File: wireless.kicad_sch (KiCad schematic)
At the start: 36 parts, among them J301 J_TC2030-IDC, Q301 Q_SOT23_NPN, Q302 Q_SOT23_NPN, U301 U_ATGM336H-5N31, U302 U_ESP32-C3-MINI-1U-N4, U303 U_AT2659, U304 U_RA-01S

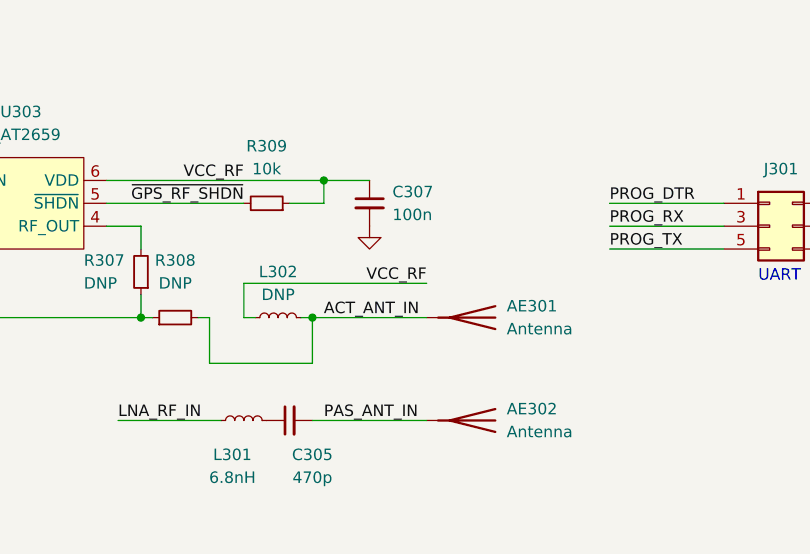
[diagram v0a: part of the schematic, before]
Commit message: production: prepare for fab
Signed-off-by: Connor Rigby <connorr@hey.com>
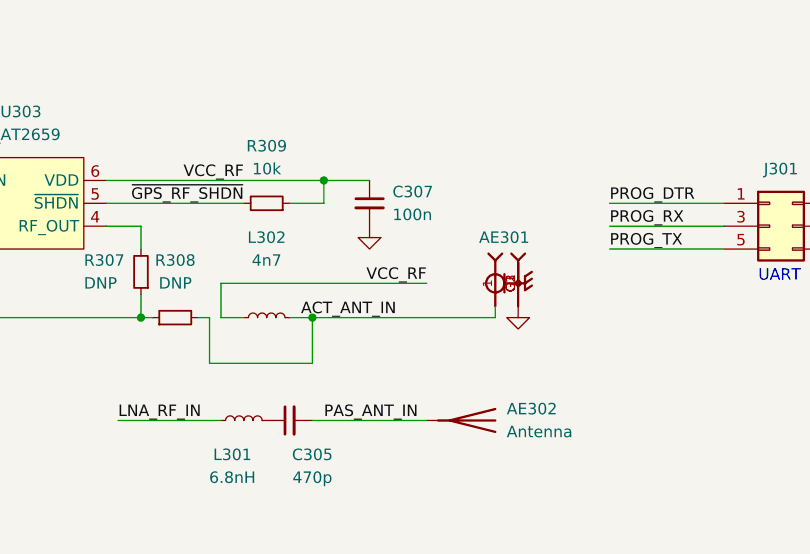
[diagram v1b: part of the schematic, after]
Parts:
- AE301: value Antenna -> 20579-001E; footprint (none) -> BOM:IPEX_20579-001E; symbol Device:Antenna -> BOM:20579-001E; LCSC (none) -> C2987683; MANUFACTURER (none) -> I-PEX; MPN (none) -> IPEX-4
- AE302, C305, C307, L301, R307, R309, U303: now left out of the parts list
- L302: value L_0402_DNP -> L_4n7; symbol BOM:L_0402_DNP -> BOM:L_4n7; Inductance DNP -> 4n7; LCSC (none) -> C13595; MPN (none) -> SDCL1005C4N7STDF
- U302: LCSC C2911374 -> C3013922; MPN ESP32-C3-MINI-1U-N4 -> ESP32-C3-MINI-1U-H4
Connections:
- net GND: now also AE301.G1, AE301.G2, AE301.G3
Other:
- moved on the sheet: L302
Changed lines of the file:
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@@
     (stroke (width 0) (type default) (color 0 0 0 0))
   )
-  (wire (pts (xy 137.16 144.78) (xy 135.89 144.78))
+  (wire (pts (xy 135.89 144.78) (xy 133.35 144.78))
     (stroke (width 0) (type default) (color 0 0 0 0))
   )
@@
     (stroke (width 0) (type default) (color 0 0 0 0))
   )
+  (wire (pts (xy 163.83 143.51) (xy 163.83 144.78))
+    (stroke (width 0) (type default) (color 0 0 0 0))
+  )
   (wire (pts (xy 243.84 67.31) (xy 260.35 67.31))
     (stroke (width 0) (type default) (color 0 0 0 0))
@@
     (stroke (width 0) (type default) (color 0 0 0 0))
   )
-  (wire (pts (xy 142.24 144.78) (xy 143.51 144.78))
+  (wire (pts (xy 140.97 144.78) (xy 143.51 144.78))
     (stroke (width 0) (type default) (color 0 0 0 0))
   )
@@
     (stroke (width 0) (type default) (color 0 0 0 0))
   )
-  (wire (pts (xy 156.21 144.78) (xy 143.51 144.78))
-    (stroke (width 0) (type default) (color 0 0 0 0))
-  )
-  (wire (pts (xy 156.21 140.97) (xy 135.89 140.97))
+  (wire (pts (xy 143.51 144.78) (xy 163.83 144.78))
+    (stroke (width 0) (type default) (color 0 0 0 0))
+  )
+  (wire (pts (xy 156.21 140.97) (xy 133.35 140.97))
     (stroke (width 0) (type default) (color 0 0 0 0))
   )
@@
     (stroke (width 0) (type default) (color 0 0 0 0))
   )
-  (wire (pts (xy 135.89 140.97) (xy 135.89 144.78))
+  (wire (pts (xy 133.35 140.97) (xy 133.35 144.78))
     (stroke (width 0) (type default) (color 0 0 0 0))
   )
@@
     (effects (font (size 1.27 1.27)) (justify left bottom))
   )
-  (label "ACT_ANT_IN" (at 144.78 144.78 0)
+  (label "ACT_ANT_IN" (at 142.24 144.78 0)
     (effects (font (size 1.27 1.27)) (justify left bottom))
   )
@@
   )
   (symbol (lib_id "BOM:R_0402_DNP") (at 124.46 139.7 180) (unit 1)
-    (in_bom yes) (on_board yes)
+    (in_bom no) (on_board no)
     (property "Reference" "R307" (id 0) (at 118.11 138.4299 0)
       (effects (font (size 1.27 1.27)) (justify right))
@@
   )
   (symbol (lib_id "Device:Antenna") (at 161.29 156.21 270) (unit 1)
-    (in_bom yes) (on_board yes) (fields_autoplaced)
+    (in_bom no) (on_board no) (fields_autoplaced)
     (property "Reference" "AE302" (id 0) (at 165.1 154.9399 90)
       (effects (font (size 1.27 1.27)) (justify left))
@@
     )
     (property "Datasheet" "" (id 3) (at 57.15 162.56 0)
+      (effects (font (size 1.27 1.27)) hide)
+    )
+    (pin "1")
+  )
+  (symbol (lib_id "power:GND") (at 166.37 143.51 0) (unit 1)
+    (in_bom yes) (on_board yes) (fields_autoplaced)
+    (property "Reference" "#PWR0106" (id 0) (at 166.37 149.86 0)
+      (effects (font (size 1.27 1.27)) hide)
+    )
+    (property "Value" "GND" (id 1) (at 166.37 148.59 0)
+      (effects (font (size 1.27 1.27)) hide)
+    )
+    (property "Footprint" "" (id 2) (at 166.37 143.51 0)
+      (effects (font (size 1.27 1.27)) hide)
+    )
+    (property "Datasheet" "" (id 3) (at 166.37 143.51 0)
       (effects (font (size 1.27 1.27)) hide)
     )
@@
   )
   (symbol (lib_id "BOM:U_AT2659") (at 111.76 132.08 0) (unit 1)
-    (in_bom yes) (on_board yes) (fields_autoplaced)
+    (in_bom no) (on_board no) (fields_autoplaced)
     (property "Reference" "U303" (id 0) (at 111.125 121.92 0))
     (property "Value" "U_AT2659" (id 1) (at 111.125 124.46 0))
@@
       (effects (font (size 1.27 1.27)) hide)
     )
-    (property "MPN" "ESP32-C3-MINI-1U-N4" (id 4) (at 110.49 57.15 0)
-      (effects (font (size 1.27 1.27)) hide)
-    )
-    (property "LCSC" "C2911374" (id 5) (at 110.49 57.15 0)
+    (property "MPN" "ESP32-C3-MINI-1U-H4" (id 4) (at 110.49 57.15 0)
+      (effects (font (size 1.27 1.27)) hide)
+    )
+    (property "LCSC" "C3013922" (id 5) (at 110.49 57.15 0)
       (effects (font (size 1.27 1.27)) hide)
     )
@@
   )
   (symbol (lib_id "BOM:C_0402_100n") (at 149.86 132.08 0) (mirror y) (unit 1)
-    (in_bom yes) (on_board yes) (fields_autoplaced)
+    (in_bom no) (on_board no) (fields_autoplaced)
     (property "Reference" "C307" (id 0) (at 152.4 130.8162 0)
       (effects (font (size 1.27 1.27)) (justify right))
@@
     (pin "2")
   )
-  (symbol (lib_id "Device:Antenna") (at 161.29 144.78 270) (unit 1)
-    (in_bom yes) (on_board yes) (fields_autoplaced)
-    (property "Reference" "AE301" (id 0) (at 165.1 143.5099 90)
+  (symbol (lib_id "BOM:20579-001E") (at 163.83 140.97 90) (mirror x) (unit 1)
+    (in_bom yes) (on_board yes)
+    (property "Reference" "AE301" (id 0) (at 167.64 135.89 90)
       (effects (font (size 1.27 1.27)) (justify left))
     )
-    (property "Value" "Antenna" (id 1) (at 165.1 146.0499 90)
-      (effects (font (size 1.27 1.27)) (justify left))
-    )
-    (property "Footprint" "" (id 2) (at 161.29 144.78 0)
-      (effects (font (size 1.27 1.27)) hide)
-    )
-    (property "Datasheet" "~" (id 3) (at 161.29 144.78 0)
-      (effects (font (size 1.27 1.27)) hide)
-    )
-    (pin "1")
+    (property "Value" "20579-001E" (id 1) (at 170.688 136.906 0)
+      (effects (font (size 1.27 1.27)) (justify left bottom) hide)
+    )
+    (property "Footprint" "BOM:IPEX_20579-001E" (id 2) (at 163.83 140.97 0)
+      (effects (font (size 1.27 1.27)) (justify bottom) hide)
+    )
+    (property "Datasheet" "https://datasheet.lcsc.com/lcsc/2203301630_ZIISOR-IPEX-4_C2987683.pdf" (id 3) (at 163.83 140.97 0)
+      (effects (font (size 1.27 1.27)) hide)
+    )
+    (property "LCSC" "C2987683" (id 4) (at 163.83 140.97 0)
+      (effects (font (size 1.27 1.27)) hide)
+    )
+    (property "MPN" "IPEX-4" (id 5) (at 163.83 140.97 0)
+      (effects (font (size 1.27 1.27)) hide)
+    )
+    (property "MANUFACTURER" "I-PEX" (id 6) (at 163.83 140.97 0)
+      (effects (font (size 1.27 1.27)) (justify bottom) hide)
+    )
+    (pin "1")
+    (pin "G1")
+    (pin "G2")
+    (pin "G3")
   )
   (symbol (lib_id "BOM:C_0402_100n") (at 147.32 41.91 0) (unit 1)
@@
   )
   (symbol (lib_id "BOM:R_0402_10k") (at 138.43 132.08 270) (mirror x) (unit 1)
-    (in_bom yes) (on_board yes)
+    (in_bom no) (on_board no)
     (property "Reference" "R309" (id 0) (at 138.43 125.73 90))
     (property "Value" "R_0402_10k" (id 1) (at 137.414 131.318 0)
@@
   )
   (symbol (lib_id "BOM:L_6n8") (at 135.89 156.21 90) (unit 1)
-    (in_bom yes) (on_board yes)
+    (in_bom no) (on_board no)
     (property "Reference" "L301" (id 0) (at 134.62 160.02 90))
     (property "Value" "L_6n8" (id 1) (at 136.906 155.448 0)
@@
     (pin "2")
   )
-  (symbol (lib_id "BOM:L_0402_DNP") (at 139.7 144.78 90) (unit 1)
+  (symbol (lib_id "BOM:L_4n7") (at 138.43 144.78 90) (unit 1)
     (in_bom yes) (on_board yes)
-    (property "Reference" "L302" (id 0) (at 139.7 139.7 90))
-    (property "Value" "L_0402_DNP" (id 1) (at 140.716 144.018 0)
+    (property "Reference" "L302" (id 0) (at 138.43 135.89 90))
+    (property "Value" "L_4n7" (id 1) (at 139.446 144.018 0)
       (effects (font (size 1.27 1.27)) (justify left) hide)
     )
-    (property "Footprint" "Inductor_SMD:L_0402_1005Metric" (id 2) (at 139.7 144.78 0)
-      (effects (font (size 1.27 1.27)) hide)
-    )
-    (property "Datasheet" "~" (id 3) (at 139.7 144.78 0)
-      (effects (font (size 1.27 1.27)) hide)
-    )
-    (property "Inductance" "DNP" (id 4) (at 139.7 142.24 90))
-    (property "DNP" "DNP" (id 5) (at 139.7 144.78 0)
+    (property "Footprint" "Inductor_SMD:L_0402_1005Metric" (id 2) (at 138.43 144.78 0)
+      (effects (font (size 1.27 1.27)) hide)
+    )
+    (property "Datasheet" "https://datasheet.lcsc.com/lcsc/2110081230_Sunlord-SDCL1005C4N7STDF_C13595.pdf" (id 3) (at 138.43 144.78 0)
+      (effects (font (size 1.27 1.27)) hide)
+    )
+    (property "Inductance" "4n7" (id 4) (at 138.43 138.43 90))
+    (property "DNP" "DNP" (id 5) (at 138.43 144.78 0)
+      (effects (font (size 1.27 1.27)) hide)
+    )
+    (property "LCSC" "C13595" (id 6) (at 138.43 144.78 0)
+      (effects (font (size 1.27 1.27)) hide)
+    )
+    (property "MPN" "SDCL1005C4N7STDF" (id 7) (at 138.43 144.78 0)
       (effects (font (size 1.27 1.27)) hide)
     )
@@
   )
   (symbol (lib_id "BOM:C_0402_470p") (at 140.97 156.21 90) (unit 1)
-    (in_bom yes) (on_board yes)
+    (in_bom no) (on_board no)
     (property "Reference" "C305" (id 0) (at 143.51 160.02 90))
     (property "Value" "C_0402_470p" (id 1) (at 143.002 155.956 0)
